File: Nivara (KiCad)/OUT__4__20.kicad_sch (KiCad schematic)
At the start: 5 parts, among them U8 GP8303-TC50-EW

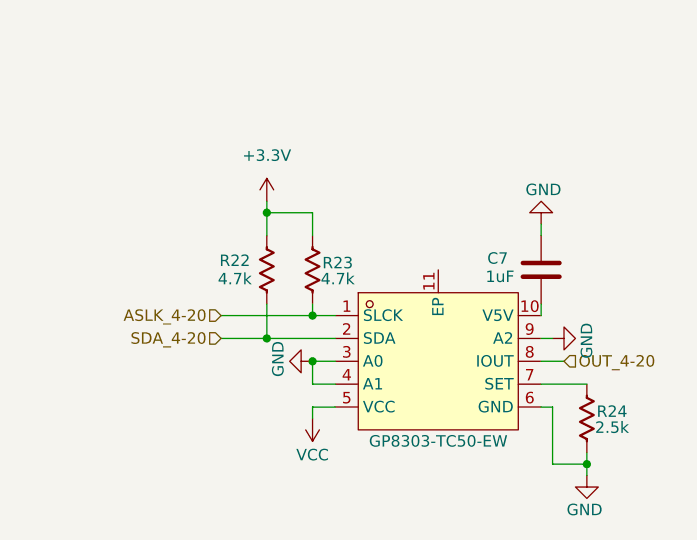
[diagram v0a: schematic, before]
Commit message: Add files via upload
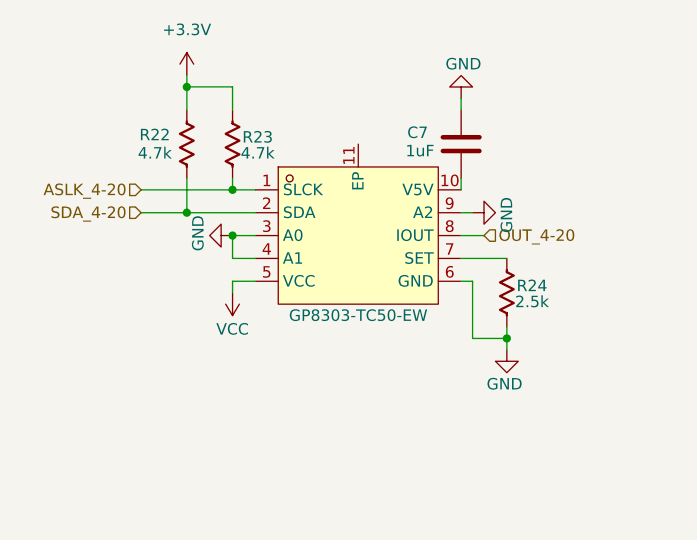
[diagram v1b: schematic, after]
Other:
- moved on the sheet: C7, R22, R23, R24
